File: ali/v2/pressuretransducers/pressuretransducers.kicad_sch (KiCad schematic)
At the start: 4 parts

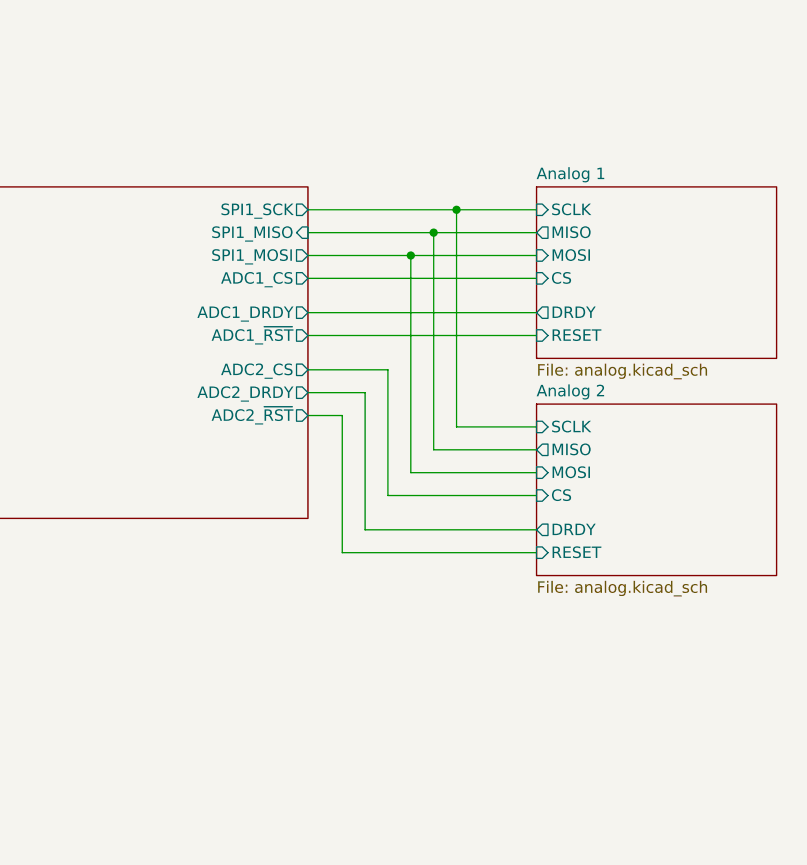
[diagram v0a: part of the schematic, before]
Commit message: Minor updates
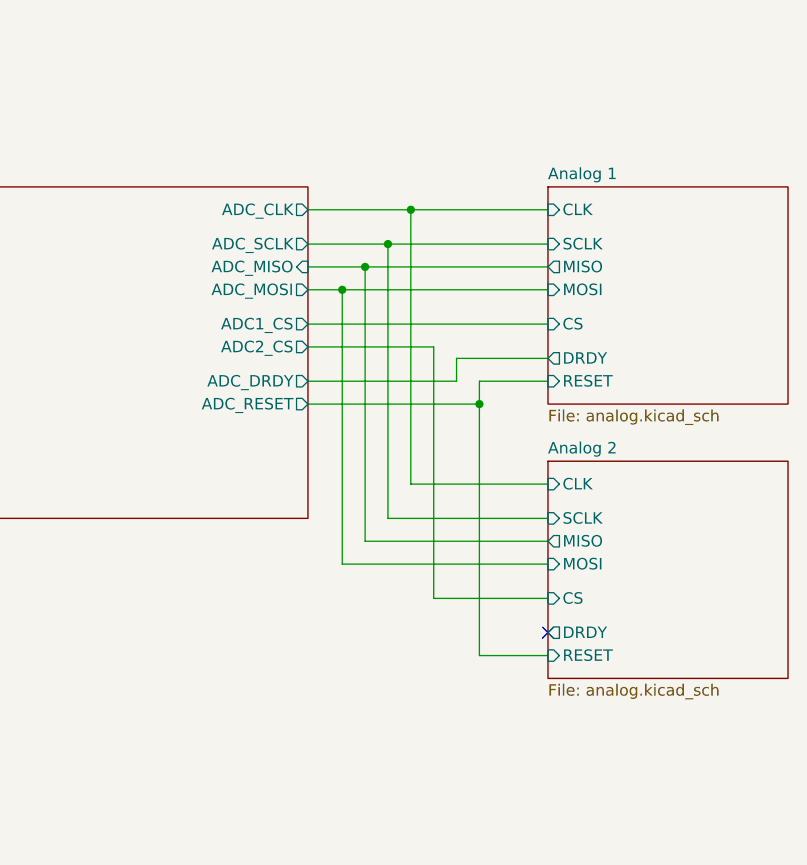
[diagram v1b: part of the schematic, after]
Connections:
- no-connect marks 0 -> 1
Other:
- sheet Analog 1 ports: added CLK; removed none
- sheet Analog 2 ports: added CLK; removed none
- sheet Microcontroller ports: added ADC_CLK, ADC_DRDY, ADC_MISO, ADC_MOSI, ADC_RESET, ADC_SCLK; removed ADC1_DRDY, ADC1_~{RST}, ADC2_DRDY, ADC2_~{RST}, SPI1_MISO, SPI1_MOSI, SPI1_SCK
